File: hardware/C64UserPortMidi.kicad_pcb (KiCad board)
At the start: 2 copper layers, 48 x 47 mm, 16 parts, among them J1 C64-UserPort, J2 MIDI IN DIN-5, J3 AVR-ISP-6, U1 ATtiny13A-PU, U2 6N138, U3 74HC595

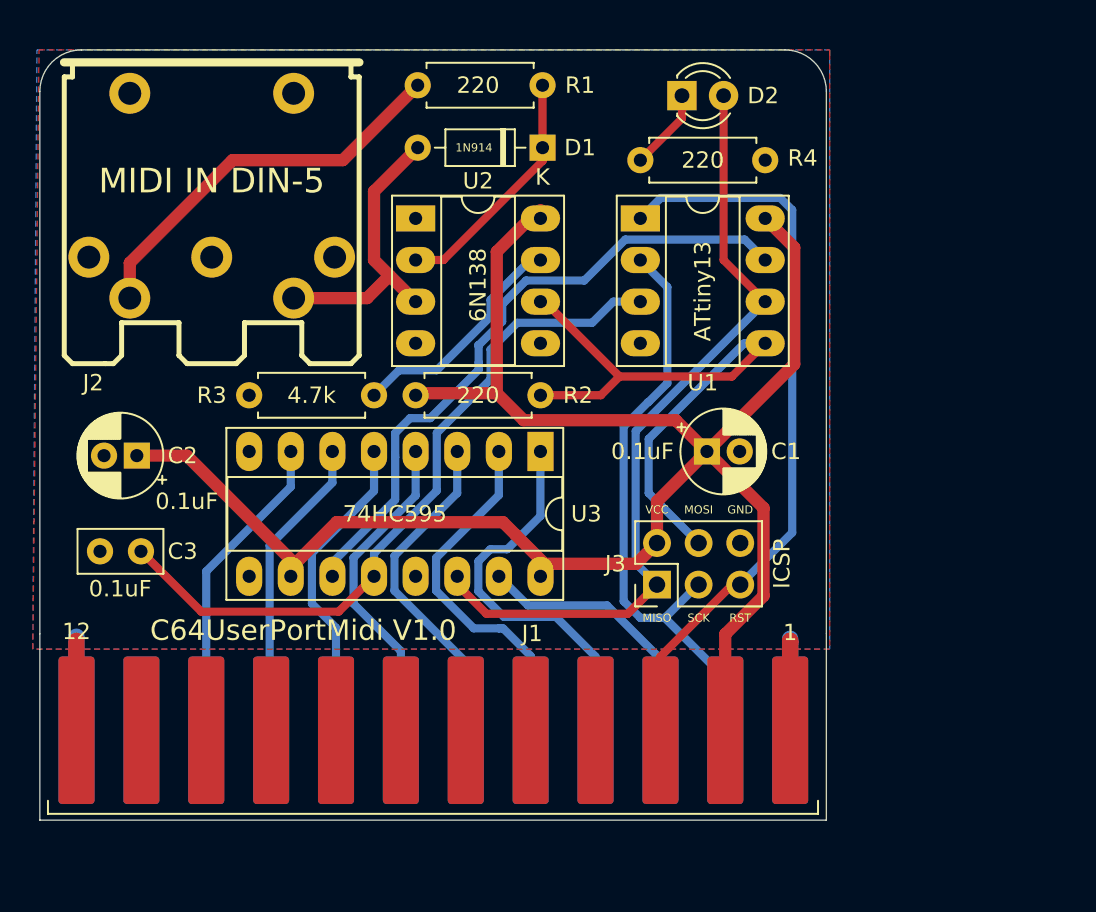
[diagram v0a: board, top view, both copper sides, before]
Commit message: New hardware design update. Version 1.0 Revision A.
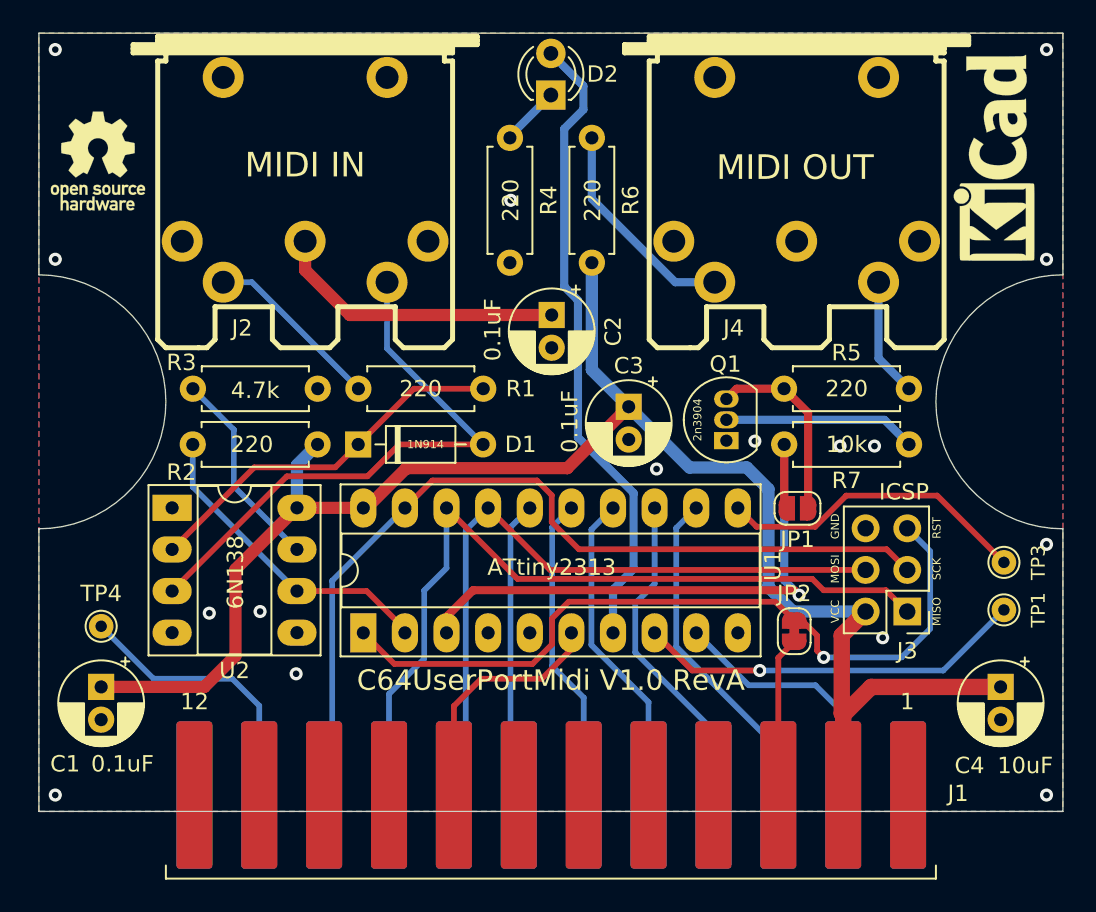
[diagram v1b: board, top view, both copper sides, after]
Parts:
- removed the REF** at (112.4, 108.8)
- removed U3: 74HC595, Package_DIP:DIP-16_W7.62mm_Socket_LongPads
- added C4: 10uF, Capacitor_THT:CP_Radial_D5.0mm_P2.00mm, F.Cu at (165.5, 127.4)
- added J4: MIDI OUT, Video Connectors:din-5, F.Cu at (153.1, 97.2)
- added JP1: MIDI Output Bypass, Jumper:SolderJumper-2_P1.3mm_Open_RoundedPad1.0x1.5mm, F.Cu at (153.1, 116.5)
- added JP2: RST Bypass, Jumper:SolderJumper-2_P1.3mm_Bridged_RoundedPad1.0x1.5mm, F.Cu at (152.9, 124.0)
- added Q1: 2N3904, Package_TO_SOT_THT:TO-92_Inline, F.Cu at (148.8, 112.4)
- added R5: 220, Resistor_THT:R_Axial_DIN0207_L6.3mm_D2.5mm_P7.62mm_Horizontal, F.Cu at (159.9, 109.2)
- added R6: 220, Resistor_THT:R_Axial_DIN0207_L6.3mm_D2.5mm_P7.62mm_Horizontal, F.Cu at (140.6, 93.9)
- added R7: 10k, Resistor_THT:R_Axial_DIN0207_L6.3mm_D2.5mm_P7.62mm_Horizontal, F.Cu at (159.9, 112.6)
- added REF**: OSHW-Logo_5.7x6mm_SilkScreen, Symbol:OSHW-Logo_5.7x6mm_SilkScreen, F.Cu at (110.4, 95.3)
- added REF**: KiCad-Logo_5mm_SilkScreen, Symbol:KiCad-Logo_5mm_SilkScreen, F.Cu at (165.6, 95.1)
- added REF**: WEEE-Logo_4.2x6mm_SilkScreen, Symbol:WEEE-Logo_4.2x6mm_SilkScreen, B.Cu at (165.4, 95.3)
- added TP1: PD4, TestPoint:TestPoint_THTPad_D1.5mm_Drill0.7mm, F.Cu at (165.7, 122.7)
- added TP3: PD6, TestPoint:TestPoint_THTPad_D1.5mm_Drill0.7mm, F.Cu at (165.7, 119.8)
- added TP4: PA2, TestPoint:TestPoint_THTPad_D1.5mm_Drill0.7mm, F.Cu at (110.6, 123.7)
- C3: footprint Capacitor_THT:C_Disc_D5.0mm_W2.5mm_P2.50mm -> Capacitor_THT:CP_Radial_D5.0mm_P2.00mm
- J2: value MIDI IN DIN-5 -> MIDI IN
- U1: value ATtiny13A-PU -> ATtiny2313-20P; footprint Package_DIP:DIP-8_W7.62mm_Socket_LongPads -> Package_DIP:DIP-20_W7.62mm_Socket_LongPads
- moved C1 39.7 mm to (110.6, 127.4), turned to -90 degrees
- moved C3 31.1 mm to (142.8, 110.3), turned to -90 degrees
- moved U1 30.4 mm to (126.6, 124.1), turned to 90 degrees
- moved C2 26.7 mm to (138.1, 104.7), turned to -90 degrees
- moved U2 23.1 mm to (114.9, 116.5)
- moved D1 21.3 mm to (126.3, 112.6), turned to 0 degrees
- moved R1 18.9 mm to (126.3, 109.2)
- moved J3 15.4 mm to (159.8, 122.8), turned to 180 degrees
- moved R3 11.1 mm to (116.2, 109.2), turned to 0 degrees
- moved J1 8.21 mm to (159.8, 134.0)
- moved R4 8.08 mm to (135.6, 93.9), turned to -90 degrees
- moved D2 8.00 mm to (138.1, 91.3), turned to 90 degrees
- moved R2 6.69 mm to (123.8, 112.6), turned to 180 degrees
- moved J2 5.78 mm to (123.0, 97.2)
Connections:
- C2 pad 1: VCC -> Net-(C2-Pad1)
- C3 pad 1: LATCH -> VCC
- D2 pad 2: DATA -> Net-(D2-Pad2)
- J1 pad 10: Net-(J1-Pad10) -> unconnected-(J1-Pad10)
- J1 pad 11: Net-(J1-Pad11) -> unconnected-(J1-Pad11)
- J1 pad 3: ~{RST} -> Net-(J1-Pad3)
- J1 pad 4: Net-(J1-Pad4) -> unconnected-(J1-Pad4)
- J1 pad 5: Net-(J1-Pad5) -> unconnected-(J1-Pad5)
- J1 pad 6: Net-(J1-Pad6) -> unconnected-(J1-Pad6)
- J1 pad 7: Net-(J1-Pad7) -> unconnected-(J1-Pad7)
- J1 pad 8: Net-(J1-Pad8) -> RECV
- J1 pad 9: Net-(J1-Pad9) -> unconnected-(J1-Pad9)
- J1 pad B: FLAG -> LATCH
- J1 pad J: /D5 -> MOSI
- J1 pad K: /D6 -> MISO
- J1 pad L: /D7 -> SCK
- J2 pad 1: Net-(J2-Pad1) -> unconnected-(J2-Pad1)
- J2 pad 2: Net-(J2-Pad2) -> Net-(C2-Pad1)
- J2 pad 3: Net-(J2-Pad3) -> unconnected-(J2-Pad3)
- J3 pad 1: DATA -> MISO
- J3 pad 3: FLAG -> SCK
- J3 pad 4: RX -> MOSI
- U1 pad 2: FLAG -> RX
- U1 pad 3: LATCH -> TX
- U1 pad 4: GND -> unconnected-(U1-Pad4)
- U1 pad 5: RX -> unconnected-(U1-Pad5)
- U1 pad 6: DATA -> RECV
- U1 pad 7: CLOCK -> Net-(D2-Pad2)
- U1 pad 8: VCC -> Net-(TP1-Pad1)
- U2 pad 1: Net-(U2-Pad1) -> GND
- U2 pad 4: Net-(U2-Pad4) -> GND
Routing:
- net SCK: track 0.00 -> 54.1 mm
- net MISO: track 0.00 -> 49.7 mm
- net DATA: track 48.9 -> 0.00 mm
- net MOSI: track 0.00 -> 43.0 mm
- net CLOCK: track 40.1 -> 0.00 mm
- net Net-(D2-Pad2): track 0.00 -> 38.9 mm
- net FLAG: track 37.4 -> 0.00 mm
- net TX: track 0.00 -> 36.8 mm, vias 0 -> 1
- net LATCH: track 43.8 -> 16.0 mm
- net Net-(TP1-Pad1): track 0.00 -> 23.8 mm, vias 0 -> 1
- net GND: track 22.4 -> 0.00 mm, vias 0 -> 16
- net RX: track 38.9 -> 19.4 mm
- net /D5: track 19.2 -> 0.00 mm
- net Net-(TP3-Pad1): track 0.00 -> 19.2 mm
- net /D7: track 19.2 -> 0.00 mm
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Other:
- board size 48 x 47 mm -> 62.5 x 47.5 mm
- board text added: "10k"
- board text added: "10uF"
- board text added: "2n3904"
- board text added: "ATtiny2313"
- board text added: "C64UserPortMidi V1.0 RevA"
- board text added: "Created By: D Cooper Dalrymple 12-2022 dcdalrymple.com"
- board text removed: "74HC595"
- board text removed: "ATtiny13"
- board text removed: "C64UserPortMidi V1.0"
- board text removed: "Created By: D Cooper Dalrymple 2021 dcdalrymple.com"
